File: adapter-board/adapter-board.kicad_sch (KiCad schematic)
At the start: 9 parts, among them J1 Conn_01x02_Socket, J2 Conn_01x05_Pin, J3 Conn_01x01_Socket, J4 Conn_01x04_Socket, J5 Conn_01x04_Socket, U1 XIAO ESP32C3

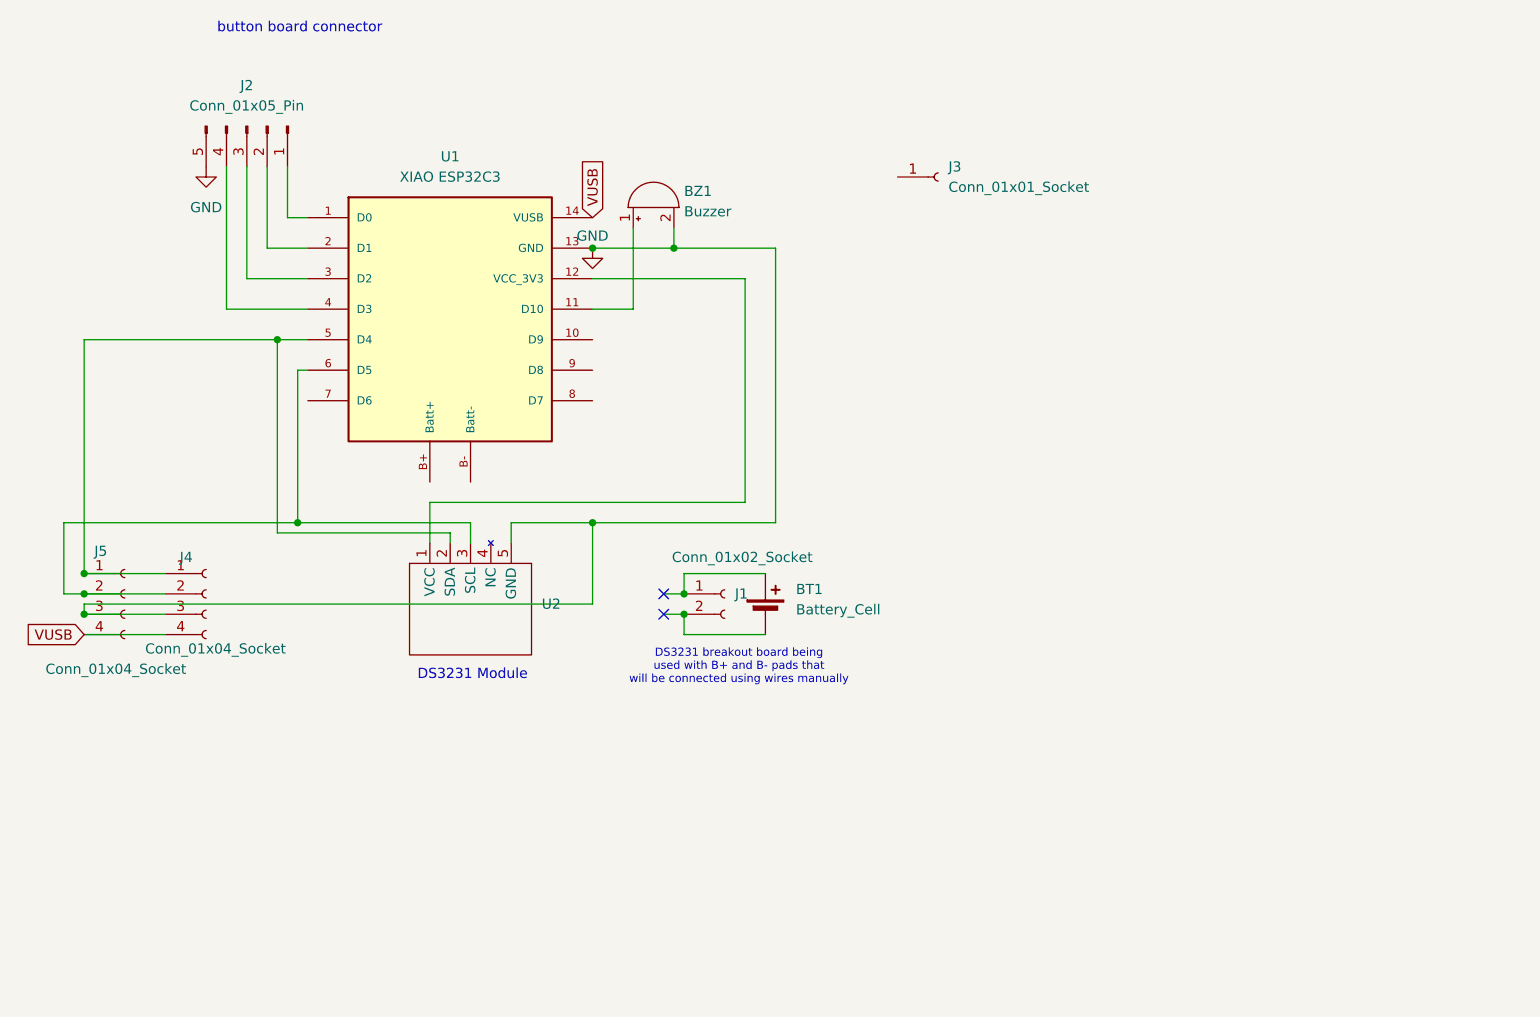
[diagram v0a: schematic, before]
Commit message: feat: PCB updates
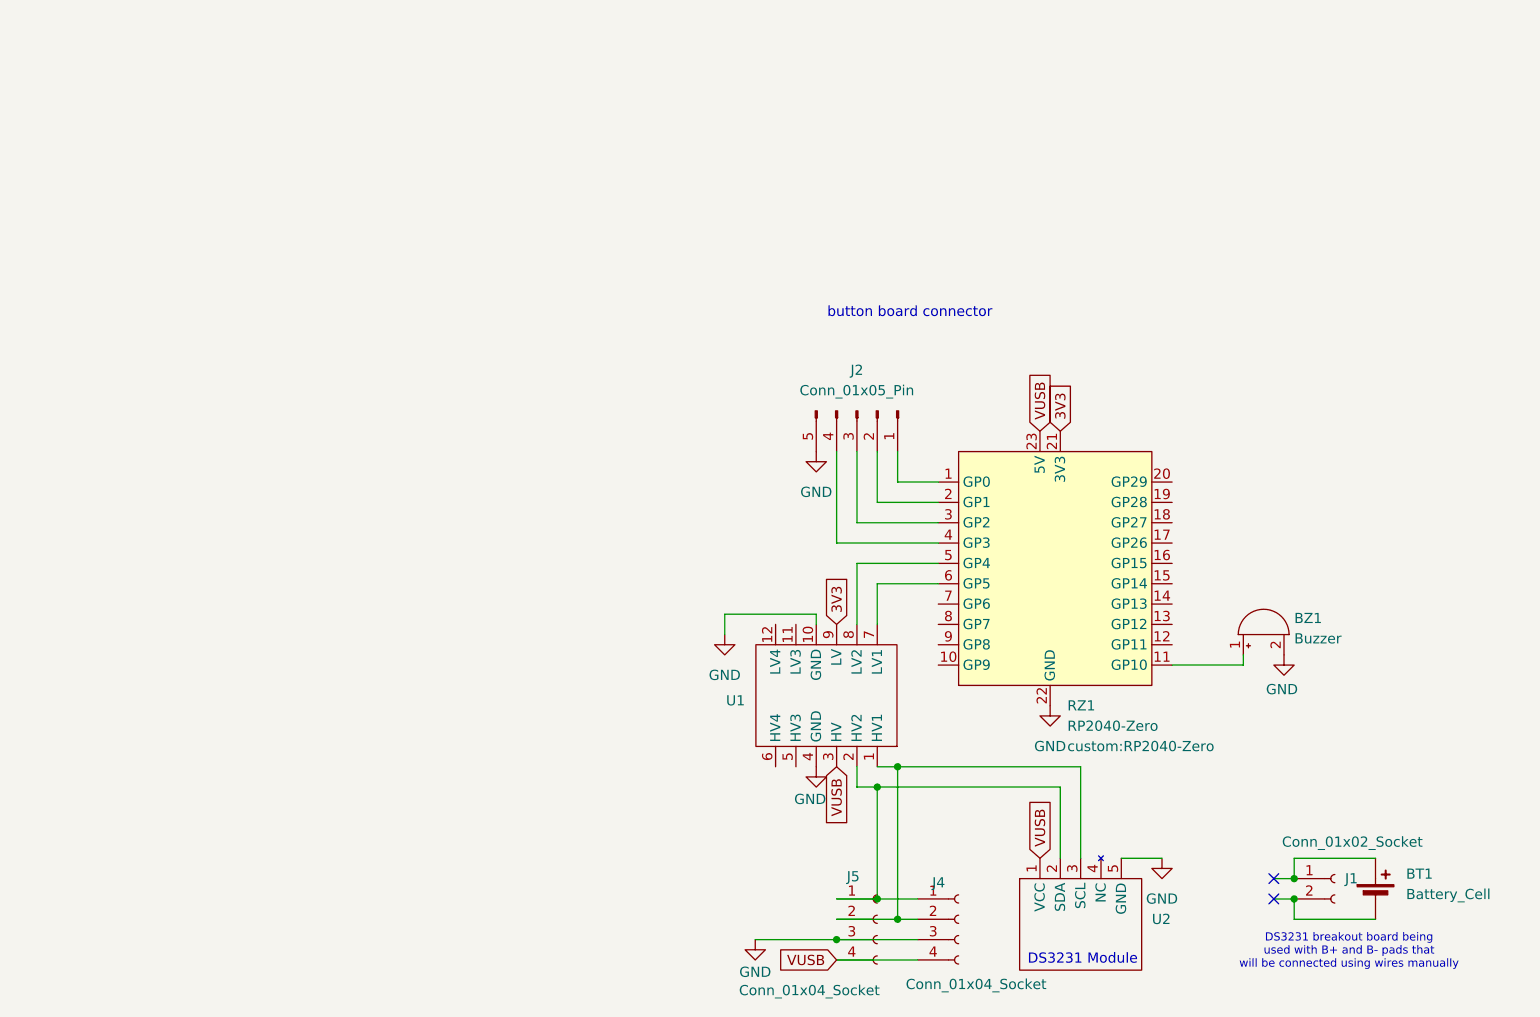
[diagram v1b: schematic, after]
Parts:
- removed J3: Conn_01x01_Socket, custom:PinMatrix05x10P2.54, symbol Connector:Conn_01x01_Socket
- removed U1: XIAO ESP32C3, xiao_esp32c3:xiao_esp32c3, symbol xiao_esp32c3:XIAO ESP32C3
- added RZ1: RP2040-Zero, custom:RP2040-Zero, symbol custom:RP2040-Zero
- added U1: ~, custom:Generic-Level-Shifter, symbol custom:Generic-Level-Shifter
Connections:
- net GND: now also RZ1.22 (GND), U1.10 (GND), U1.4 (GND)
- net VUSB: now also U2.1 (VCC), RZ1.23 (5V), U1.3 (HV)
- net at J4.1 (Pin_1), J5.1 (Pin_1), U2.2 (SDA): now also U1.2 (HV2)
- net at J4.2 (Pin_2), J5.2 (Pin_2), U2.3 (SCL): now also U1.1 (HV1)
- net at BZ1.1 (+): now also RZ1.11 (GP10)
- net at J2.1 (Pin_1): now also RZ1.1 (GP0)
- net at J2.2 (Pin_2): now also RZ1.2 (GP1)
- net at J2.3 (Pin_3): now also RZ1.3 (GP2)
- net at J2.4 (Pin_4): now also RZ1.4 (GP3)
- new net: RZ1.5 (GP4), U1.8 (LV2)
- new net: RZ1.6 (GP5), U1.7 (LV1)
- new net 3V3: RZ1.21 (3V3), U1.9 (LV)
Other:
- moved on the sheet: BT1, BZ1, J1, J2, J4, J5, U2
